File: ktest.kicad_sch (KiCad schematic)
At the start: 0 parts

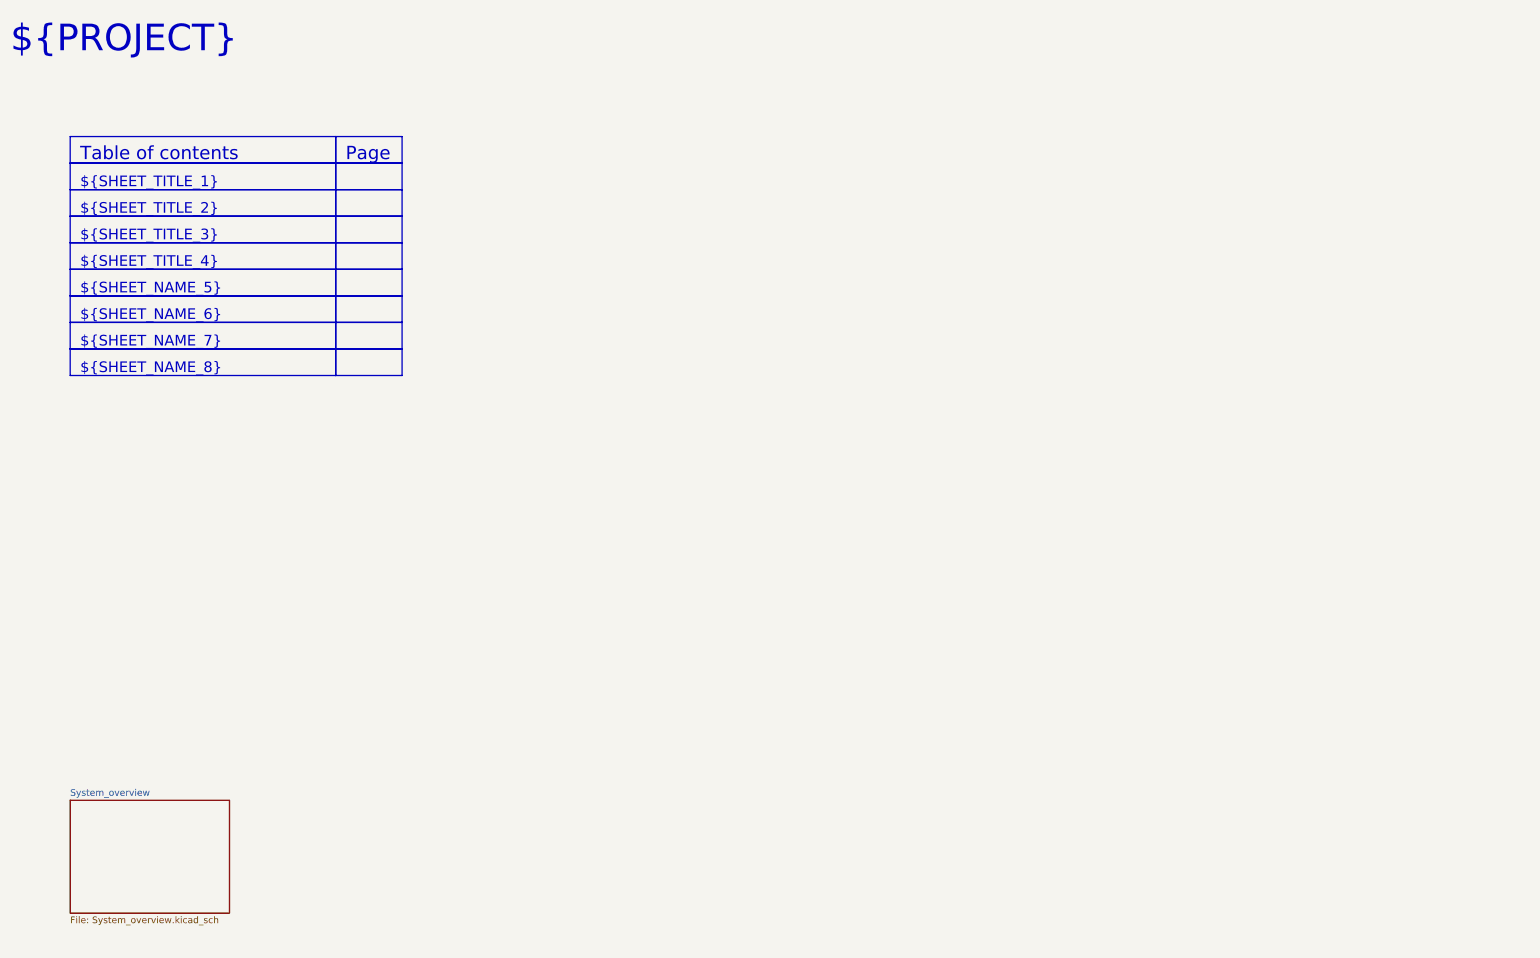
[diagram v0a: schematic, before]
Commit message: system overview and interfaces done
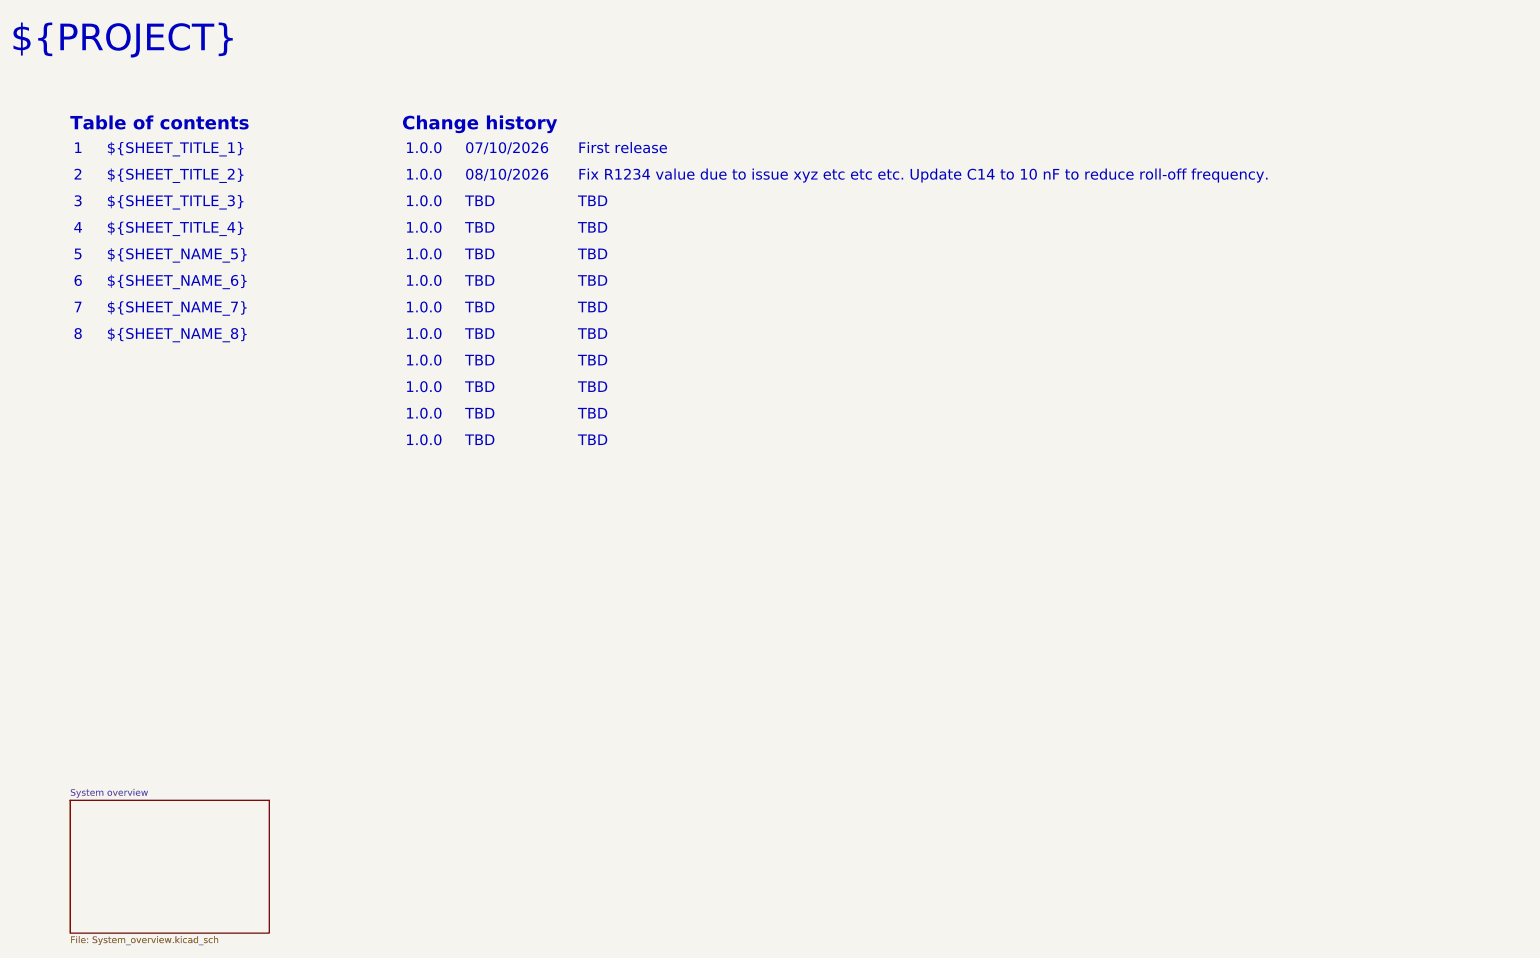
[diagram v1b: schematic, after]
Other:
- sheet System_overview renamed System overview
- note added: "07/10/2026"
- note added: "08/10/2026"
- note added: "1"
- note added: "1.0.0"
- note added: "2"
- note added: "3"
- note added: "4"
- note added: "5"
- note added: "6"
- note added: "7"
- note added: "8"
- note added: "Change history"
- note added: "First release"
- note added: "Fix R1234 value due to issue xyz etc etc etc. Update C14 to 10 nF to reduce roll-off frequency."
- note added: "TBD"
- note removed: "Page"

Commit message: testing green mask
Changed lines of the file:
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@@
 				(face "DejaVu Sans")
 				(size 5.08 5.08)
-				(thickness 0.3175)
 				(color 0 0 0 1)
 			)
